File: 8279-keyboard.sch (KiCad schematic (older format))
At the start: 27 parts, among them SW10 SW_Push, SW11 SW_Push, SW12 SW_Push, SW13 SW_Push, SW14 SW_Push, SW15 SW_Push, SW16 SW_Push, SW17 SW_Push, SW18 SW_Push, SW19 SW_Push, SW20 SW_Push, SW21 SW_Push, SW22 SW_Push, SW23 SW_Push, SW24 SW_Push, SW3 SW_Push, SW4 SW_Push, SW5 SW_Push, SW6 SW_Push, SW7 SW_Push, SW8 SW_Push, SW9 SW_Push, U15 pkd8279, U16 74LS138

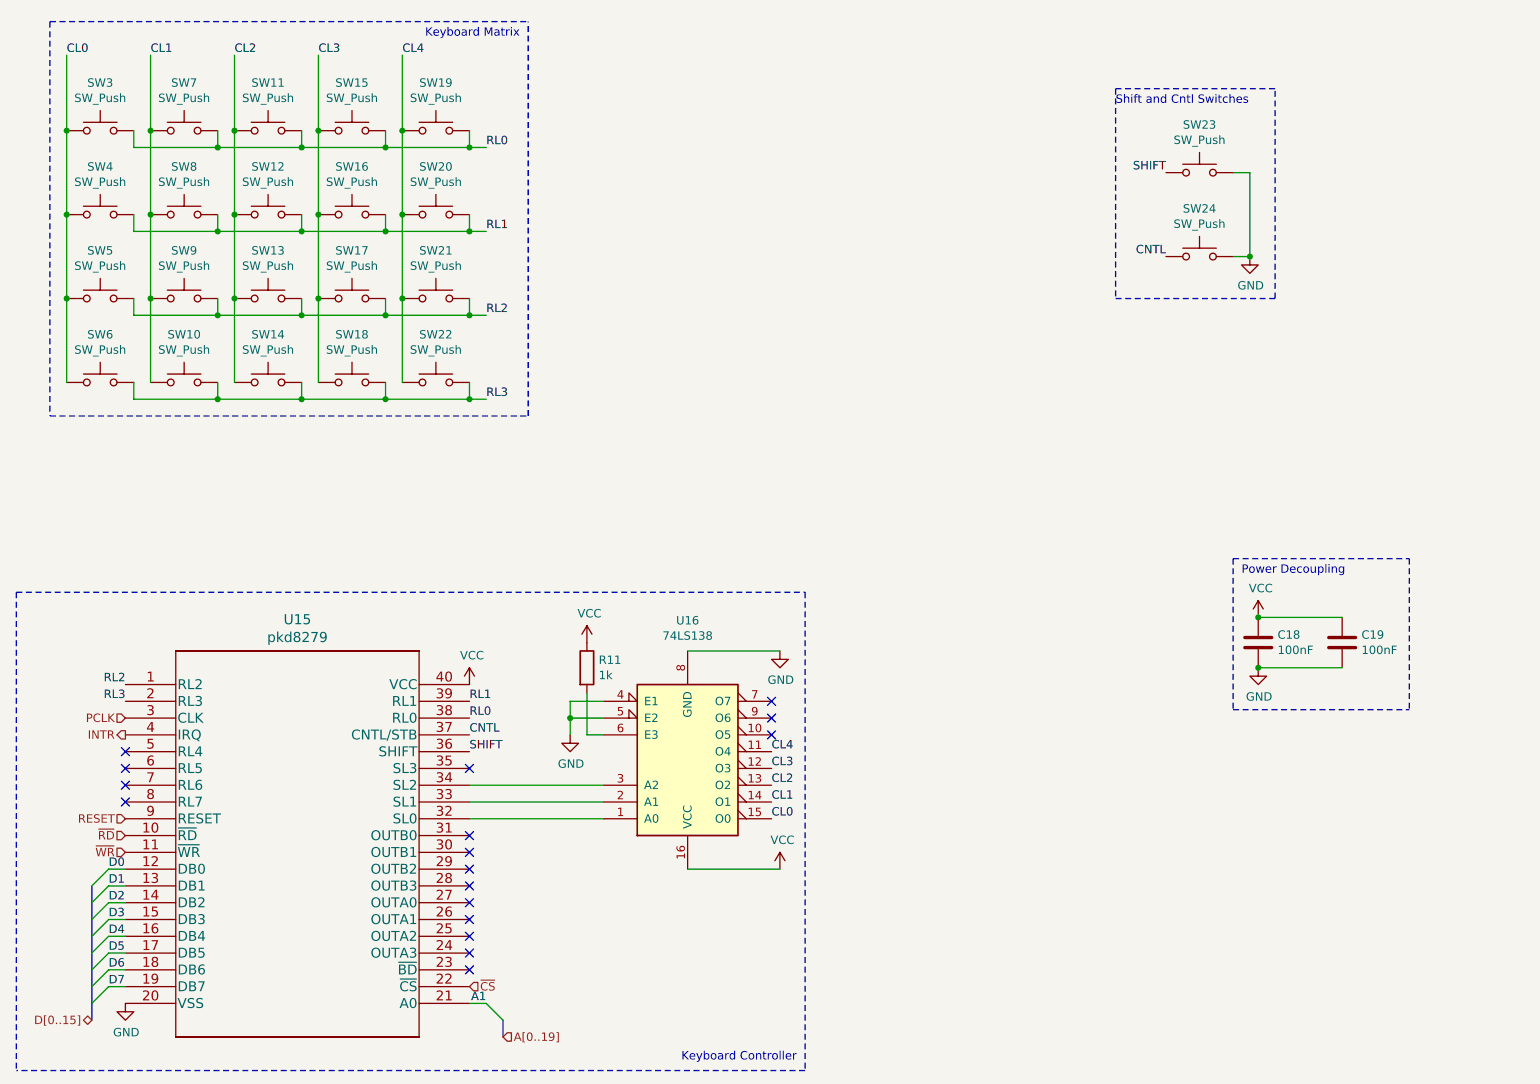
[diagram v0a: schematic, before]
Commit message: assign footprints and edits
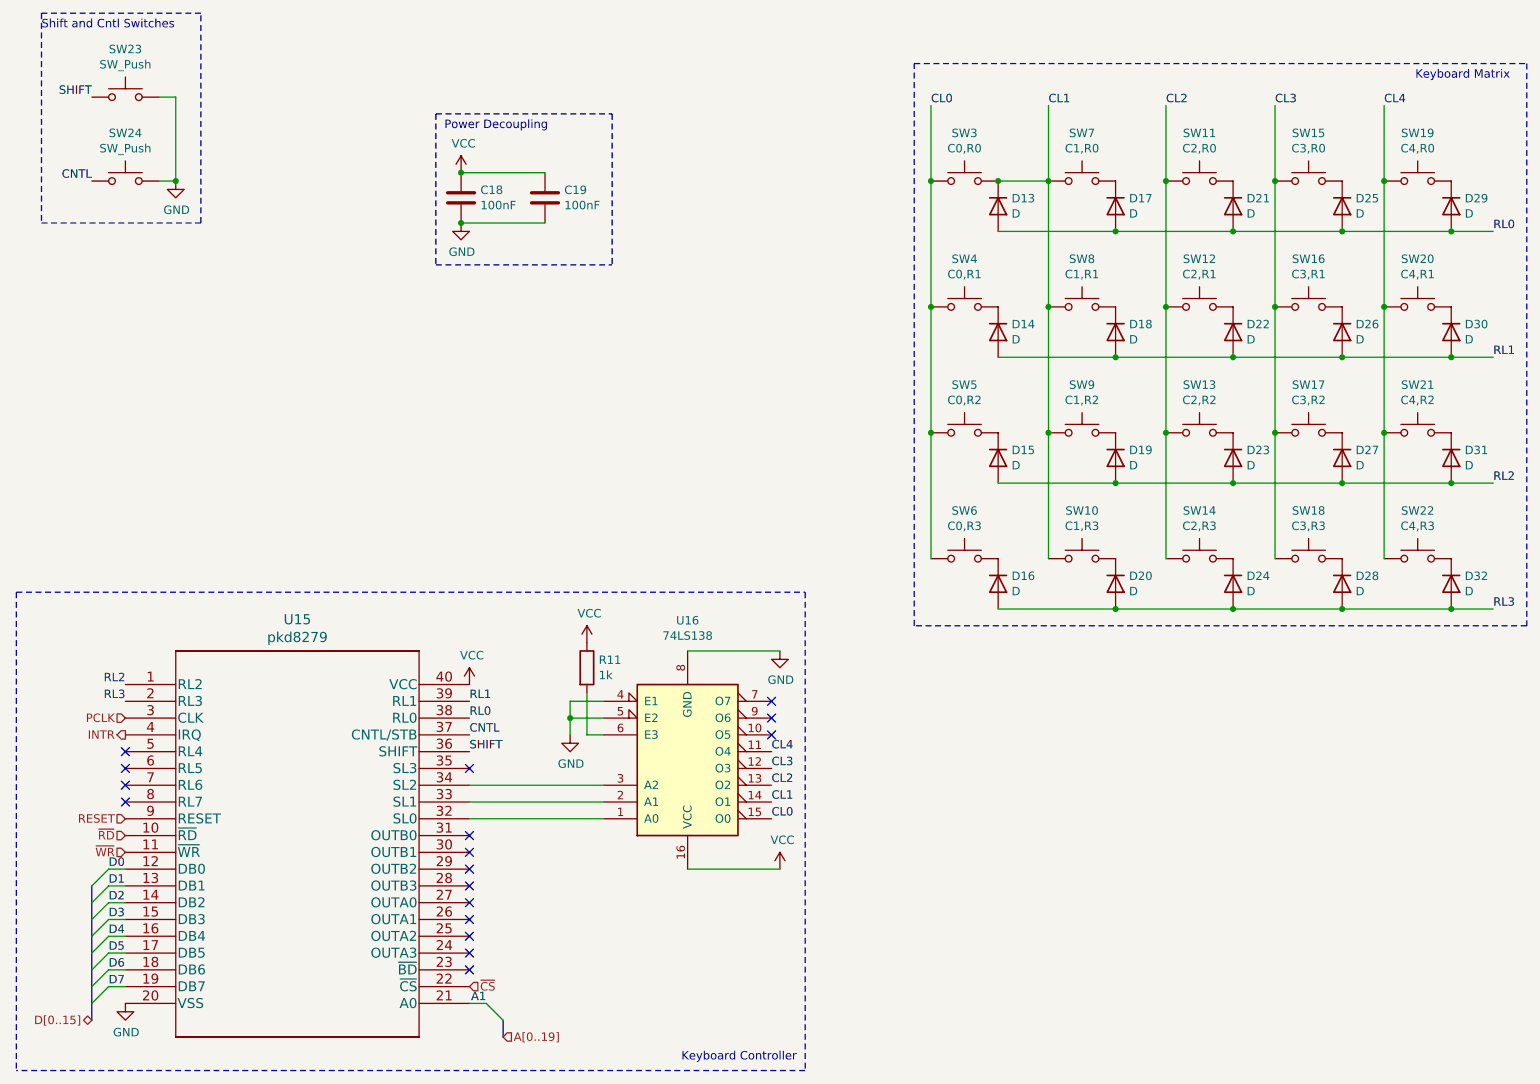
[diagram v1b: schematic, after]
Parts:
- added D13, D14, D15, D16, D17, D18, D19, D20, D21, D22, D23, D24, D25, D26, D27, D28, D29, D30, D31, D32: D, Diode_THT:D_DO-35_SOD27_P7.62mm_Horizontal, symbol Device:D
- SW10: value SW_Push -> C1,R3
- SW11: value SW_Push -> C2,R0
- SW12: value SW_Push -> C2,R1
- SW13: value SW_Push -> C2,R2
- SW14: value SW_Push -> C2,R3
- SW15: value SW_Push -> C3,R0
- SW16: value SW_Push -> C3,R1
- SW17: value SW_Push -> C3,R2
- SW18: value SW_Push -> C3,R3
- SW19: value SW_Push -> C4,R0
- SW20: value SW_Push -> C4,R1
- SW21: value SW_Push -> C4,R2
- SW22: value SW_Push -> C4,R3
- SW3: value SW_Push -> C0,R0
- SW4: value SW_Push -> C0,R1
- SW5: value SW_Push -> C0,R2
- SW6: value SW_Push -> C0,R3
- SW7: value SW_Push -> C1,R0
- SW8: value SW_Push -> C1,R1
- SW9: value SW_Push -> C1,R2
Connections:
- net CL1: now also SW3.2, D13.1 (K)
- net RL0: now also D13.2 (A), D17.2 (A), D21.2 (A), D25.2 (A), D29.2 (A); no longer SW11.2, SW15.2, SW19.2, SW3.2, SW7.2
- net RL1: now also D14.2 (A), D18.2 (A), D22.2 (A), D26.2 (A), D30.2 (A); no longer SW12.2, SW16.2, SW20.2, SW4.2, SW8.2
- net RL2: now also D15.2 (A), D19.2 (A), D23.2 (A), D27.2 (A), D31.2 (A); no longer SW13.2, SW17.2, SW21.2, SW5.2, SW9.2
- net RL3: now also D16.2 (A), D20.2 (A), D24.2 (A), D28.2 (A), D32.2 (A); no longer SW10.2, SW14.2, SW18.2, SW22.2, SW6.2
- new net: D17.1 (K), SW7.2
- new net: D21.1 (K), SW11.2
- new net: D25.1 (K), SW15.2
- new net: D29.1 (K), SW19.2
- new net: D14.1 (K), SW4.2
- new net: D18.1 (K), SW8.2
- new net: D22.1 (K), SW12.2
- new net: D26.1 (K), SW16.2
- new net: D30.1 (K), SW20.2
- new net: D15.1 (K), SW5.2
- new net: D19.1 (K), SW9.2
- new net: D23.1 (K), SW13.2
- new net: D27.1 (K), SW17.2
- new net: D31.1 (K), SW21.2
- new net: D16.1 (K), SW6.2
- new net: D20.1 (K), SW10.2
- new net: D24.1 (K), SW14.2
- new net: D28.1 (K), SW18.2
- new net: D32.1 (K), SW22.2
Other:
- moved on the sheet: C18, C19, SW10, SW11, SW12, SW13, SW14, SW15, SW16, SW17, SW18, SW19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
